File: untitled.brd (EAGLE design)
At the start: 100 x 70 mm, 1 part

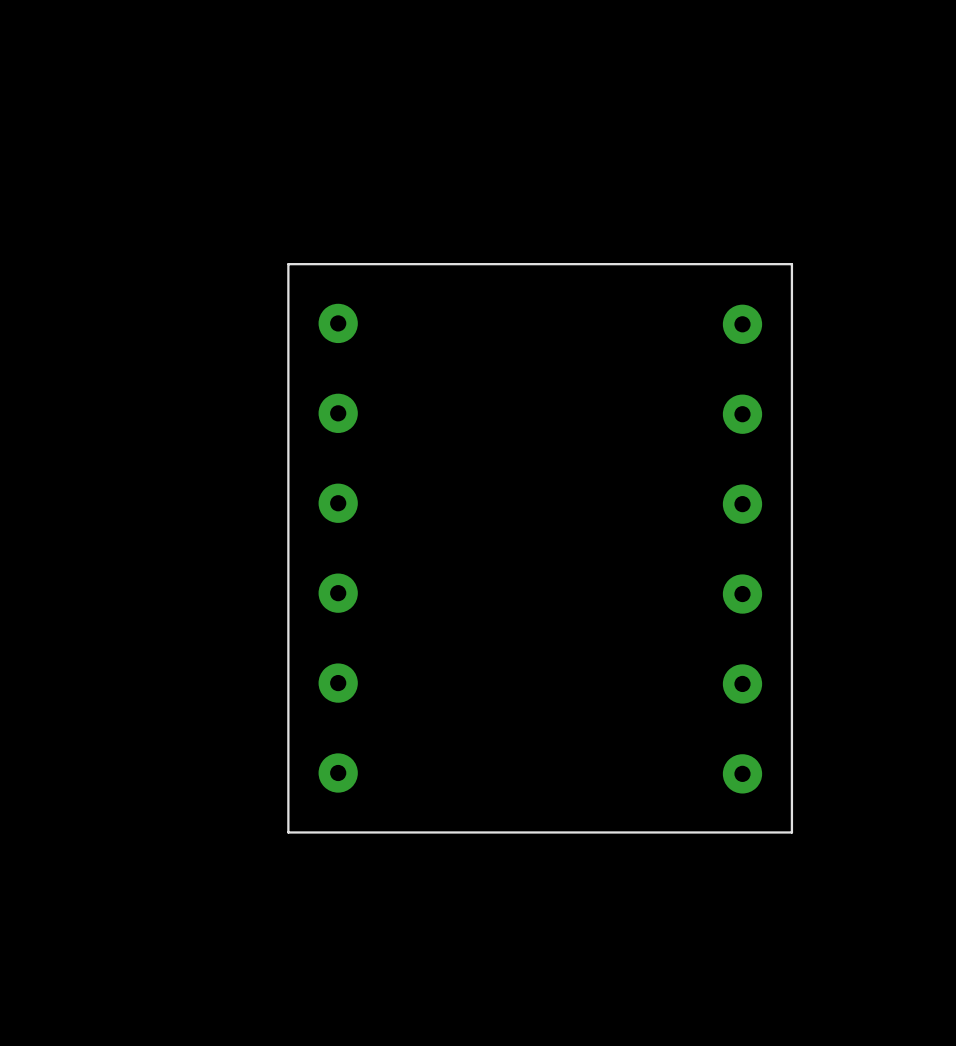
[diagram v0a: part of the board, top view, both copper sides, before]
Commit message: add
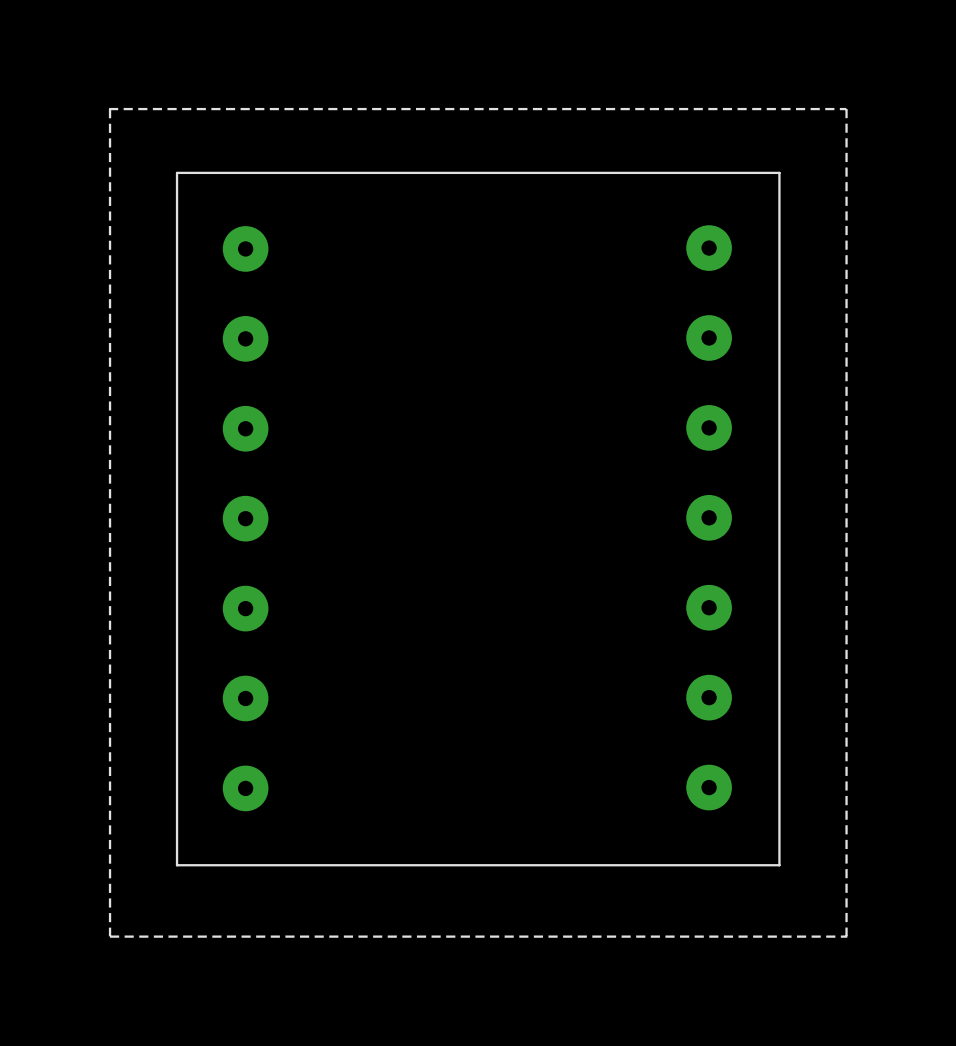
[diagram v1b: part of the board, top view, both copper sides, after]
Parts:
- removed U$1: TRANSFORMER-EE40, untitled:EE40/EI40
- added U$2: TRANSFORMER-EE40-DOWN, untitled:EE40/EI40-DOWN
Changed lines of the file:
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@@
 </autorouter>
 <elements>
-<element name="U$1" library="untitled" package="EE40/EI40" value="TRANSFORMER-EE40" x="76.51" y="34.76" smashed="yes" rot="R90"/>
+<element name="U$2" library="untitled" package="EE40/EI40-DOWN" value="TRANSFORMER-EE40-DOWN" x="73.208" y="36.477" smashed="yes"/>
 </elements>
 <signals>
